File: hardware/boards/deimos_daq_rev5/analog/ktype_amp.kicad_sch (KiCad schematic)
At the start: 12 parts, among them IC9001 INA826AIDR, J9001 AM-K-PCB

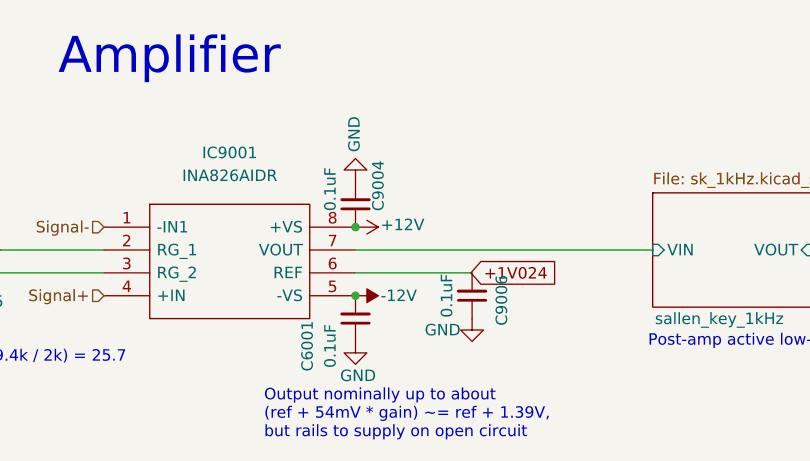
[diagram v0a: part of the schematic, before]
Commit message: restore rev5 and make this rev rev6
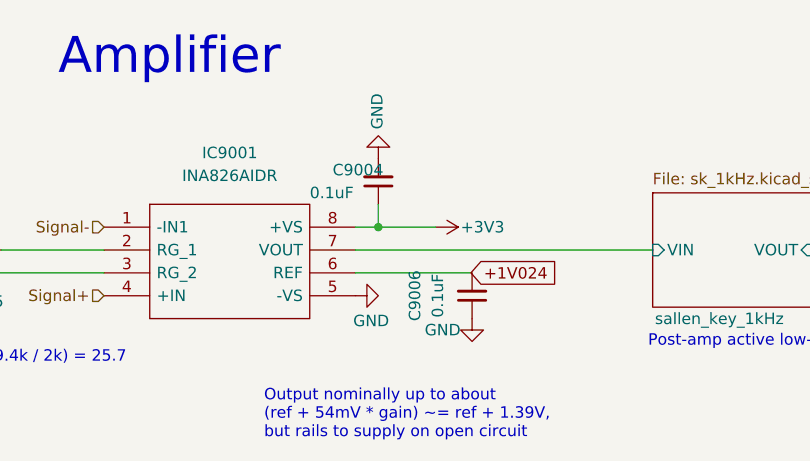
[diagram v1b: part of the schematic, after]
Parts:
- removed C6001: 0.1uF, Capacitor_SMD:C_0402_1005Metric, symbol Device:C_Small
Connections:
- net -12V is gone; now on net GND: IC9001.5 (-VS)
- net +12V renamed +3V3
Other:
- moved on the sheet: C9004
